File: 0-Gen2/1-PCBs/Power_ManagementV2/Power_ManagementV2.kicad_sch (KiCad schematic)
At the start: 86 parts, among them J1 Conn_01x02_Pin, J2 Conn_01x02_Pin, J3 Conn_01x08, J4 Conn_01x08, J5 Conn_01x02_Pin, J6 Conn_01x02_Pin, J7 USB_A_Stacked, J8 SBH11-PBPC-D10-ST-BK, Q1 MCTL160N15Y-TP, Q2 MCTL160N15Y-TP, Q3 MCTL160N15Y-TP, Q4 MCTL160N15Y-TP, Q5 MCTL160N15Y-TP, Q6 MCTL160N15Y-TP, U1 STPS5045SG-TR, U14 MCP9808_MSOP, U2 STPS5045SG-TR, U3 LTC1255CS8-PBF, U4 BA033CC0FP-E2, U5 ACS758LCB-100U-PFF-T

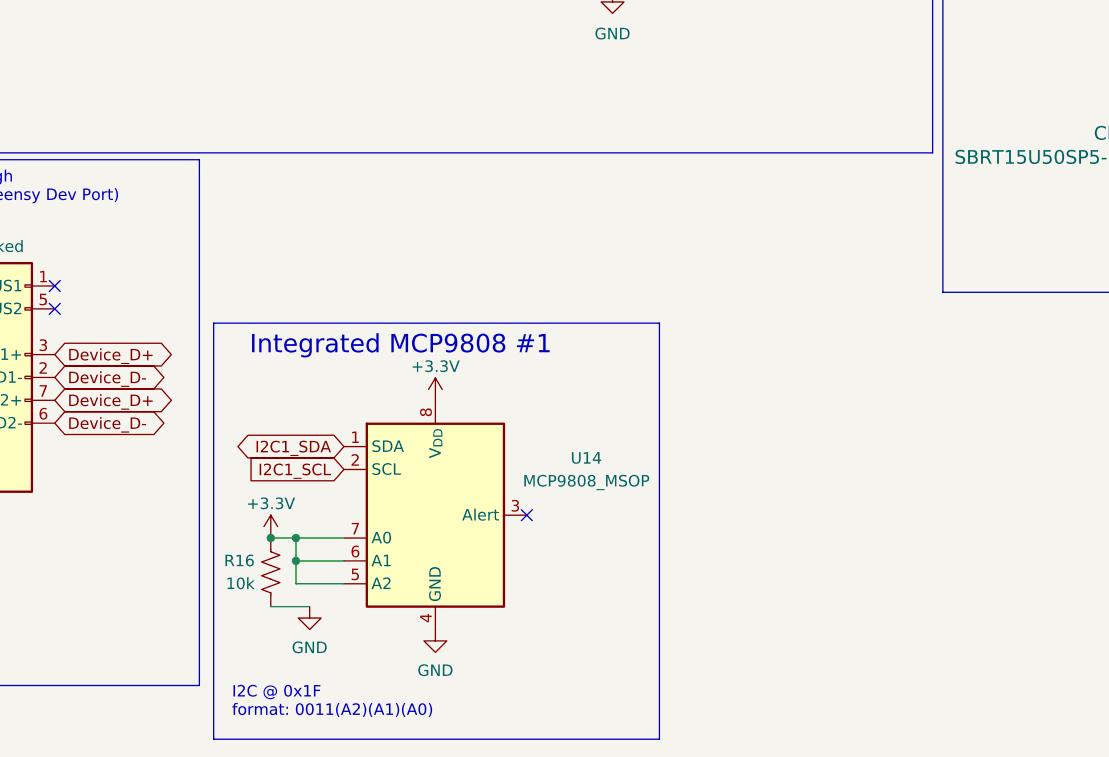
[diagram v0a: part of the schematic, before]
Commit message: done with dist
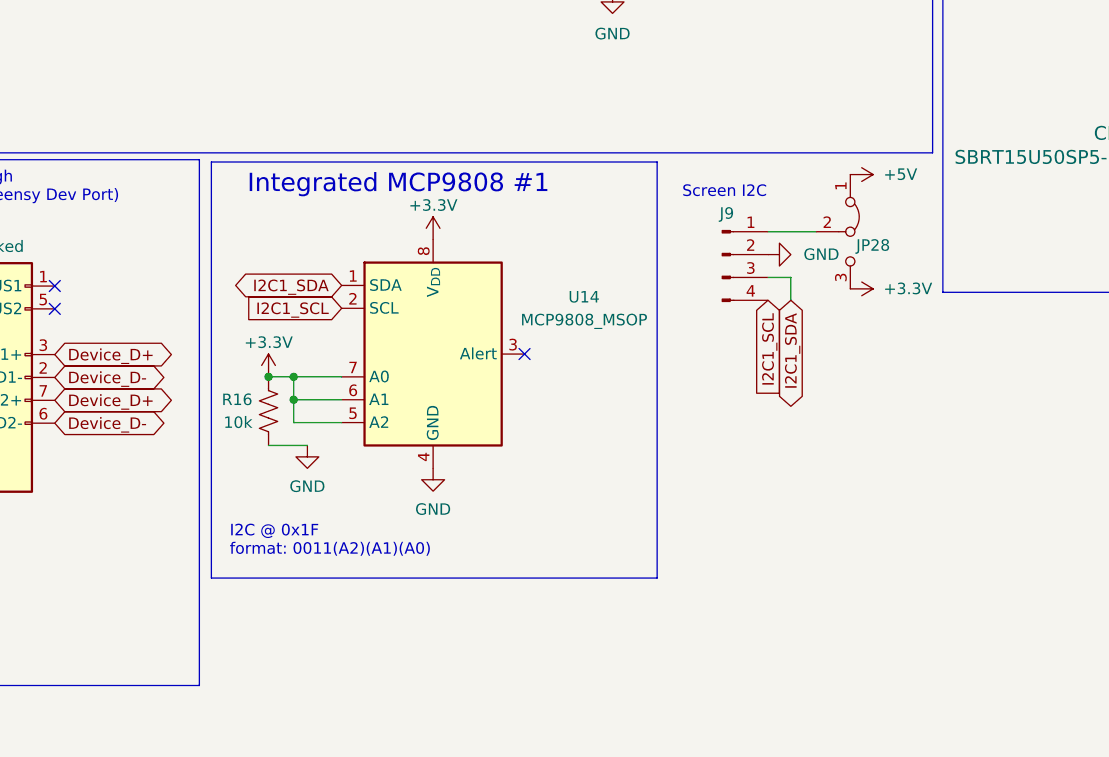
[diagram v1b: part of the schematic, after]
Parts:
- added J9: Conn_01x04_Pin, Imported_Footprints:CONN_SD-43045-008_04_MOL, symbol Connector:Conn_01x04_Pin
- added JP28: Jumper_3_Bridged12, Jumper:SolderJumper-3_P1.3mm_Bridged2Bar12_RoundedPad1.0x1.5mm, symbol Jumper:Jumper_3_Bridged12
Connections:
- net +3.3V: now also JP28.3 (B)
- net +5V: now also JP28.1 (A)
- net -BATT1: now also J9.2 (Pin_2)
- net I2C1_SCL: now also J9.4 (Pin_4)
- net I2C1_SDA: now also J9.3 (Pin_3)
- new net: J9.1 (Pin_1), JP28.2 (C)
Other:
- note added: "Screen I2C"
- moved on the sheet: R16, U14
